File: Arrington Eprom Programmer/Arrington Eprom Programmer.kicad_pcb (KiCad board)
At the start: 2 copper layers, 71.4 x 53.3 mm, 19 parts, among them J1 PGM volt in, J2 DB25_Male, SW1 SW_SPDT, U1 74LS164, U2 2716, U3 74LS299, U4 4N35

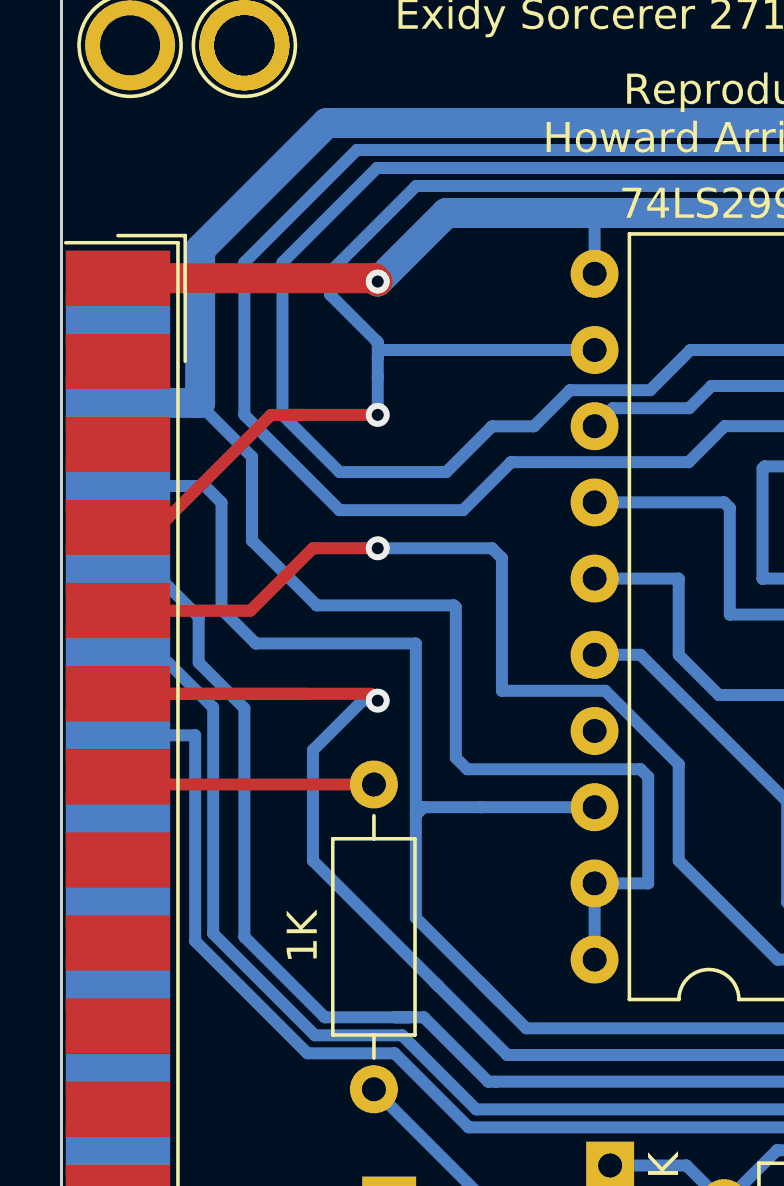
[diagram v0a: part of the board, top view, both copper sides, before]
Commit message: updated some DRC stuff
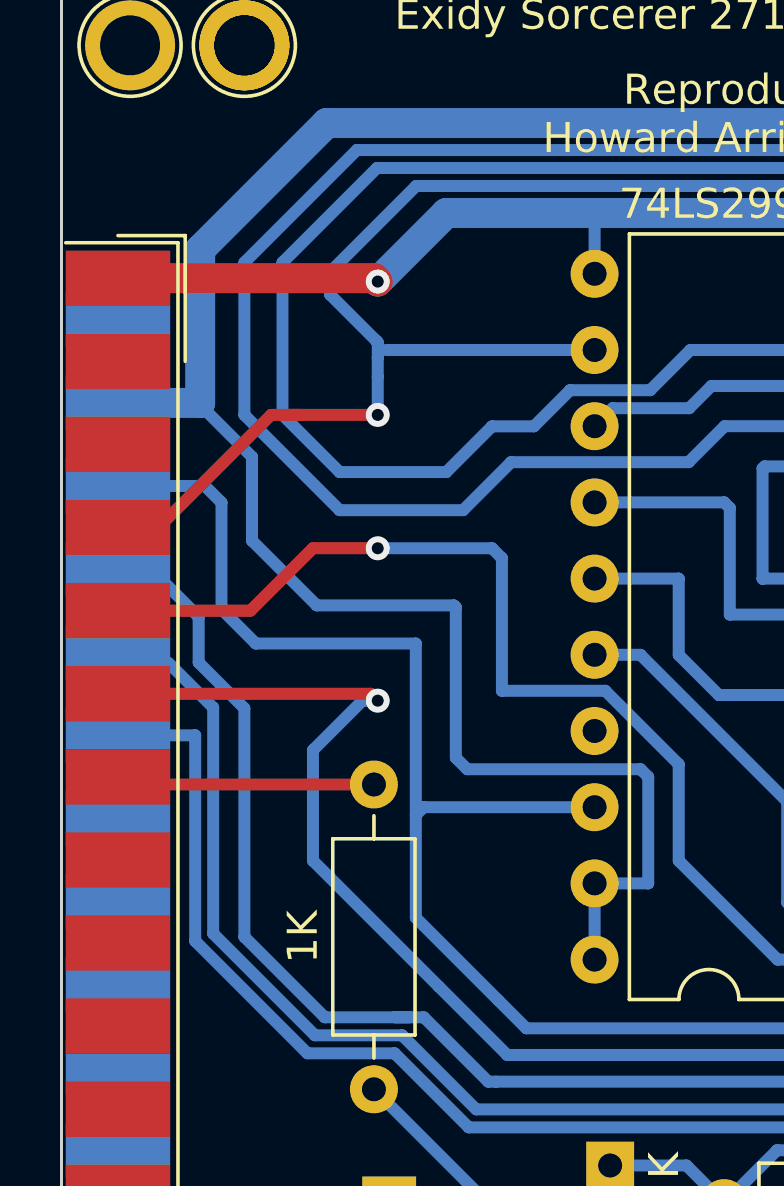
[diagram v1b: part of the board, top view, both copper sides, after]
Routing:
- net /Out5: track 54.0 -> 47.6 mm
- net /Out7: track 113.3 -> 111.0 mm
- net /Out0: track 75.3 -> 74.4 mm
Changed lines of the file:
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@@
   (via (at 95.885 86.995) (size 0.8) (drill 0.4) (layers "F.Cu" "B.Cu") (net 8))
   (segment (start 95.8265 84.5135) (end 94.2975 82.9845) (width 0.4) (layer "B.Cu") (net 8))
-  (segment (start 100.081 84.831) (end 101.6 84.831) (width 0.4) (layer "B.Cu") (net 8))
   (segment (start 151.892 106.934) (end 146.558 106.934) (width 0.4) (layer "B.Cu") (net 8))
   (segment (start 146.558 106.934) (end 145.293 105.669) (width 0.4) (layer "B.Cu") (net 8))
@@
   (segment (start 98.425 79.36448) (end 97.16552 79.36448) (width 0.4) (layer "B.Cu") (net 8))
   (segment (start 95.885 84.572) (end 95.8265 84.5135) (width 0.4) (layer "B.Cu") (net 8))
-  (segment (start 97.67352 79.36448) (end 98.425 79.36448) (width 0.4) (layer "B.Cu") (net 8))
   (segment (start 145.115634 89.154) (end 153.02448 97.062846) (width 0.4) (layer "B.Cu") (net 8))
   (segment (start 145.293 105.669) (end 142.23 105.669) (width 0.4) (layer "B.Cu") (net 8))
-  (segment (start 100.076 84.836) (end 100.081 84.831) (width 0.4) (layer "B.Cu") (net 8))
   (segment (start 129.260846 83.17448) (end 134.73648 83.17448) (width 0.4) (layer "B.Cu") (net 8))
   (segment (start 98.425 79.36448) (end 125.450846 79.36448) (width 0.4) (layer "B.Cu") (net 8))
@@
   (segment (start 99.695 91.44) (end 95.885 91.44) (width 0.4) (layer "B.Cu") (net 9))
   (segment (start 87.2265 96.29) (end 95.655 96.29) (width 0.4) (layer "F.Cu") (net 10))
-  (segment (start 87.2265 96.29) (end 93.496 96.29) (width 0.4) (layer "F.Cu") (net 10))
   (segment (start 95.655 96.29) (end 95.885 96.52) (width 0.4) (layer "F.Cu") (net 10))
   (via (at 95.885 96.52) (size 0.8) (drill 0.4) (layers "F.Cu" "B.Cu") (net 10))
-  (segment (start 97.917 106.045) (end 97.79 105.918) (width 0.4) (layer "B.Cu") (net 10))
   (segment (start 93.726 101.854) (end 93.726 98.171) (width 0.4) (layer "B.Cu") (net 10))
   (segment (start 97.917 106.045) (end 93.726 101.854) (width 0.4) (layer "B.Cu") (net 10))
@@
   (segment (start 123.444 101.854) (end 120.142 101.854) (width 0.4) (layer "B.Cu") (net 20))
   (segment (start 90.678 89.916) (end 90.127 89.365) (width 0.4) (layer "B.Cu") (net 20))
-  (segment (start 99.8855 106.4895) (end 99.314 105.918) (width 0.4) (layer "B.Cu") (net 20))
   (segment (start 114.554 107.442) (end 100.838 107.442) (width 0.4) (layer "B.Cu") (net 20))
-  (segment (start 99.319 100.071) (end 99.314 100.076) (width 0.4) (layer "B.Cu") (net 20))
   (segment (start 91.821 94.615) (end 90.678 93.472) (width 0.4) (layer "B.Cu") (net 20))
   (segment (start 97.155 94.615) (end 91.821 94.615) (width 0.4) (layer "B.Cu") (net 20))
